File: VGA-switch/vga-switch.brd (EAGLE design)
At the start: 82.2 x 63.5 mm, 15 parts, among them J1 2.1MMJACKTHM, K1 RR2A, K2 RR2A, K3 RR2A, K4 RR2A, K5 RR2A, K6 RR2A, K7 RR2A, K8 RR2A, X1 D-SUB15-HDR15RA, X2 D-SUB15-HDR15RA

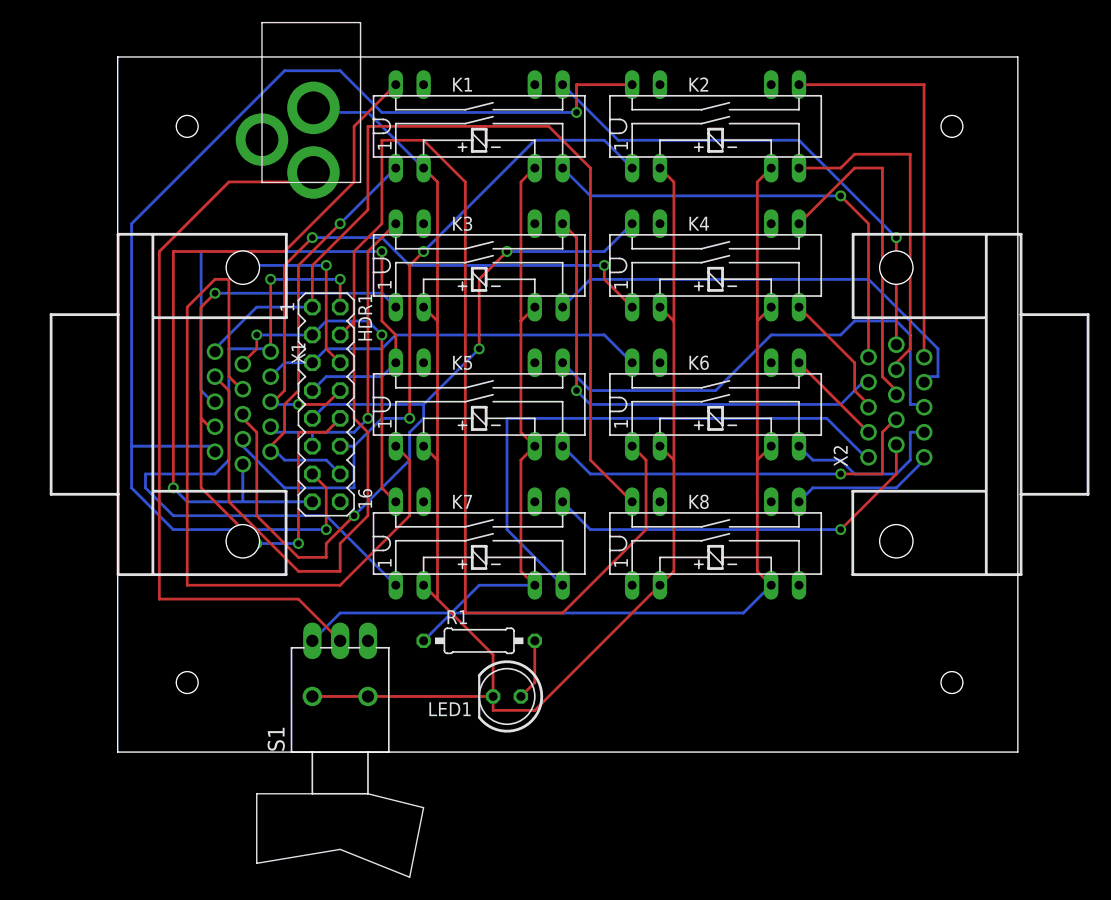
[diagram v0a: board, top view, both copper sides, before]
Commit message: board changes, layout, and logo work
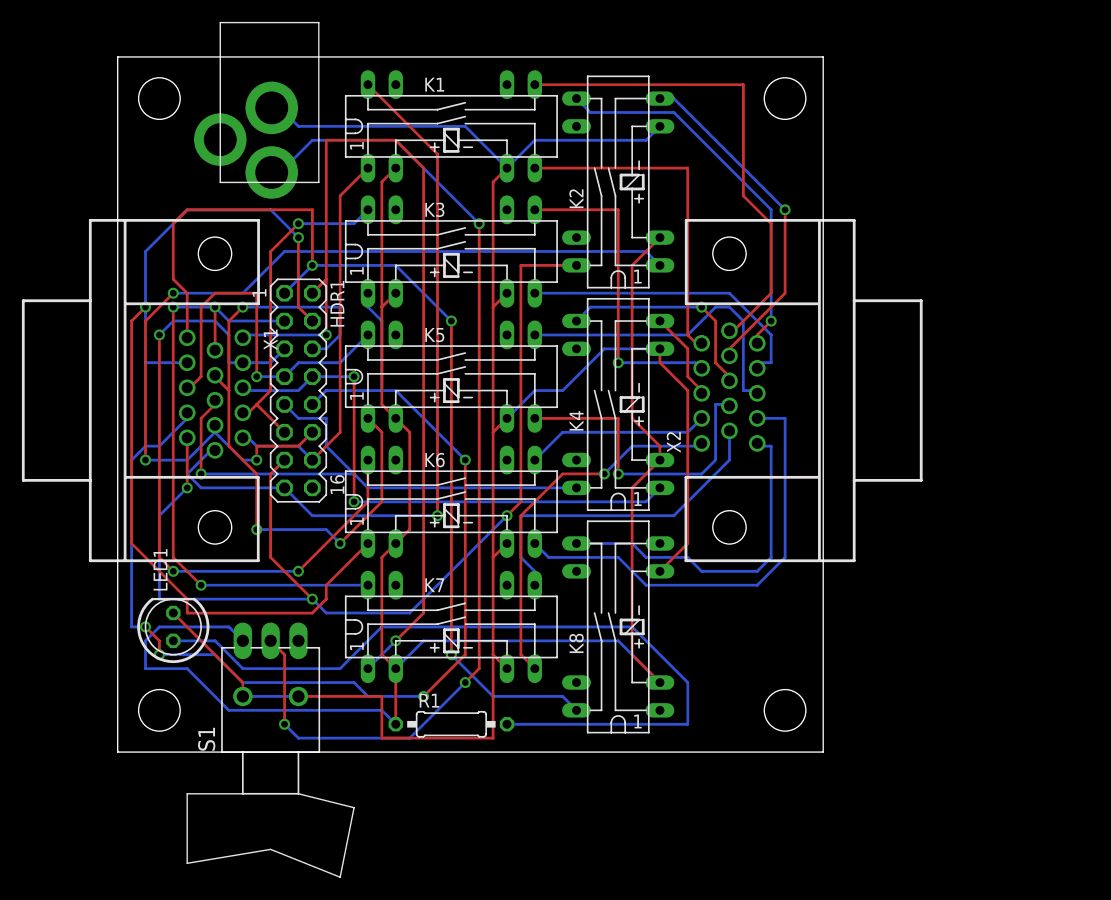
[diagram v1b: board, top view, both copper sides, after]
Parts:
- moved LED1 31.1 mm to (5.08, 11.4), turned to 90 degrees
- moved K6 25.7 mm to (30.5, 22.9)
- moved K4 15.5 mm to (45.7, 31.8), turned to 90 degrees
- moved X2 15.3 mm to (55.9, 33.0)
- moved K8 11.7 mm to (45.7, 11.4), turned to 90 degrees
- moved K2 10.2 mm to (45.7, 52.1), turned to 90 degrees
- moved K7 8.03 mm to (30.5, 11.4)
- moved R1 8.03 mm to (30.5, 2.54)
- moved S1 6.35 mm to (14.0, 5.08)
- moved J1 3.81 mm to (14.0, 62.2)
- moved K5 3.59 mm to (30.5, 34.3)
- moved HDR1 2.84 mm to (16.5, 33.0)
- moved K3 2.84 mm to (30.5, 45.7)
- moved X1 2.84 mm to (8.89, 33.0)
- moved K1 2.54 mm to (30.5, 57.1)
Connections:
- removed net N$20: K1.6, K2.6, K3.6, K4.6, K5.6, K6.6, K7.6, K8.6, R1.1, S1.3
- new net N$4: K1.2, K2.2, K3.2, K4.2, K5.2, K6.2, K7.2, K8.2, R1.1, S1.3
- net N$2: now also K1.6, K2.6, K3.6, K4.6, K5.6, K6.6, K7.6, K8.6; no longer K1.2, K2.2, K3.2, K4.2, K5.2, K6.2, K7.2, K8.2
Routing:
- net N$4: track 0.00 -> 164.8 mm
- net N$20: track 141.0 -> 0.00 mm
- net N$5: track 5.61 -> 72.0 mm
- net N$16: track 144.9 -> 89.2 mm, vias 0 -> 2
- net N$10: track 63.1 -> 102.2 mm, vias 3 -> 4
- net N$14: track 89.7 -> 60.0 mm, vias 2 -> 3
- net N$15: track 35.7 -> 61.9 mm, vias 0 -> 3
- net N$2: track 149.0 -> 174.9 mm
- net N$1: track 67.3 -> 92.9 mm, vias 0 -> 3
- net N$44: track 15.5 -> 40.7 mm
- net N$17: track 31.4 -> 56.3 mm, vias 2 -> 3
- net N$11: track 75.7 -> 52.5 mm, vias 3 -> 1
- net N$18: track 65.7 -> 85.2 mm
- net N$8: track 63.7 -> 82.6 mm, vias 2 -> 3
- net N$46: track 52.2 -> 33.9 mm, vias 0 -> 1
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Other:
- board size 82.2 x 63.5 mm -> 64.4 x 63.5 mm
